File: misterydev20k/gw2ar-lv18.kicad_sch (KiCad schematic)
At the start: 53 parts, among them J3 Jumper block, U11 LY68L6400SLIT, U5 GW2AR-LV18-QN88, U6 W25Q128JVS, U8 SY8113BADC, Y2 27MHz

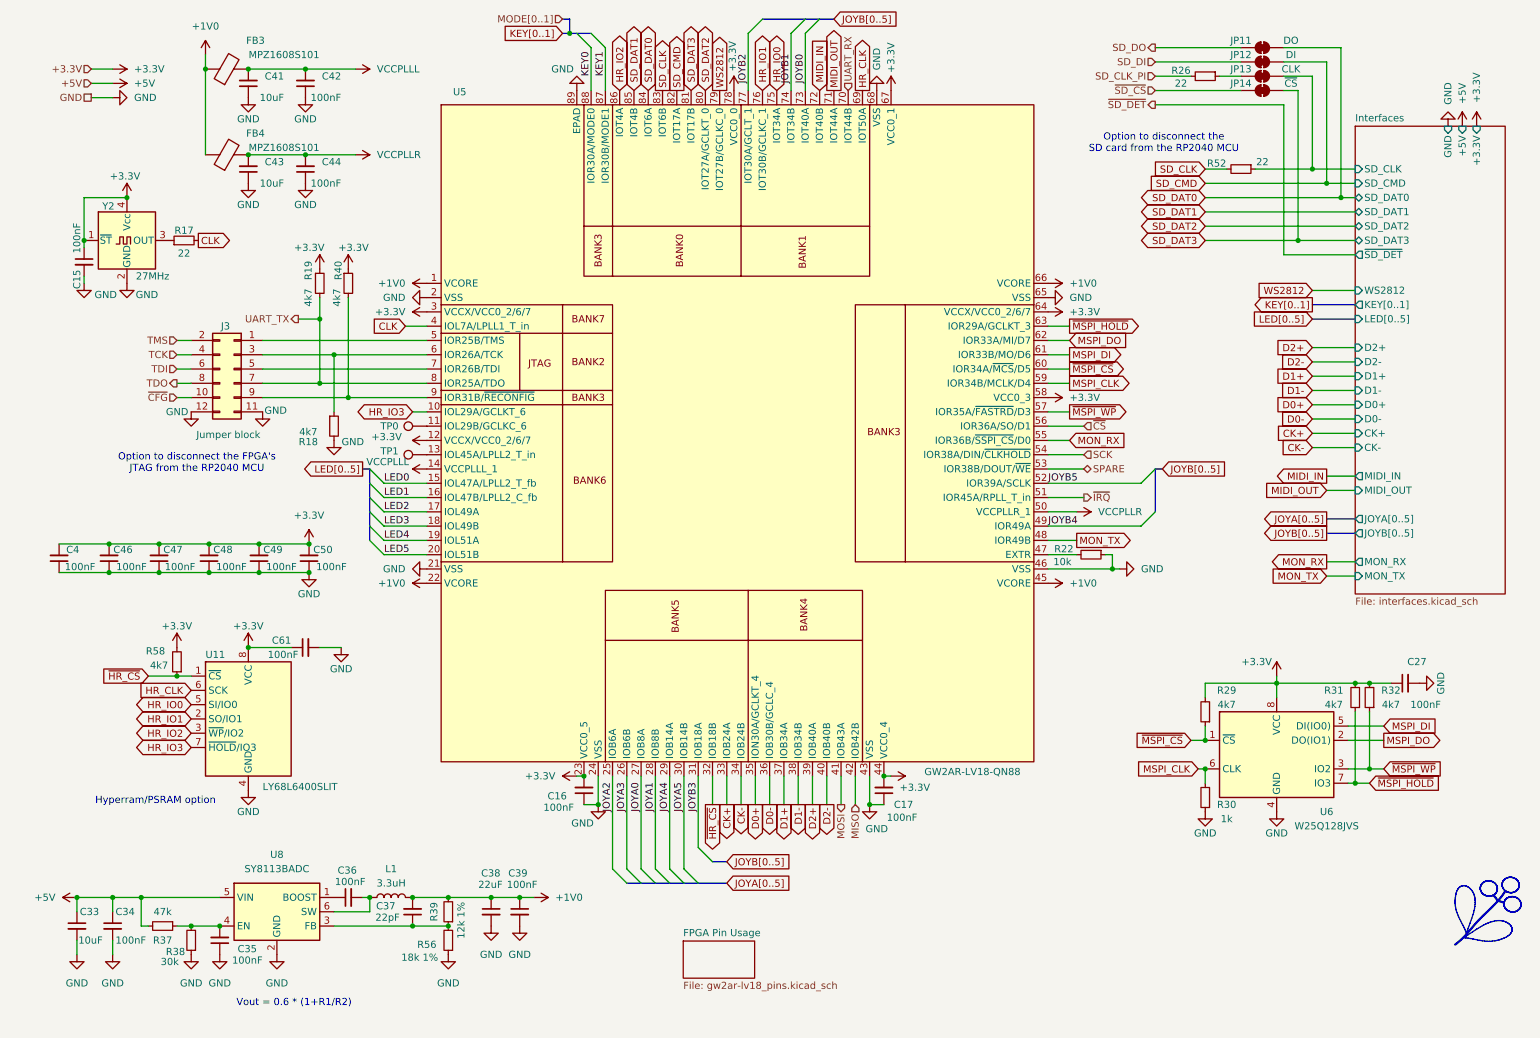
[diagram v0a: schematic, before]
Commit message: More small pcb updates
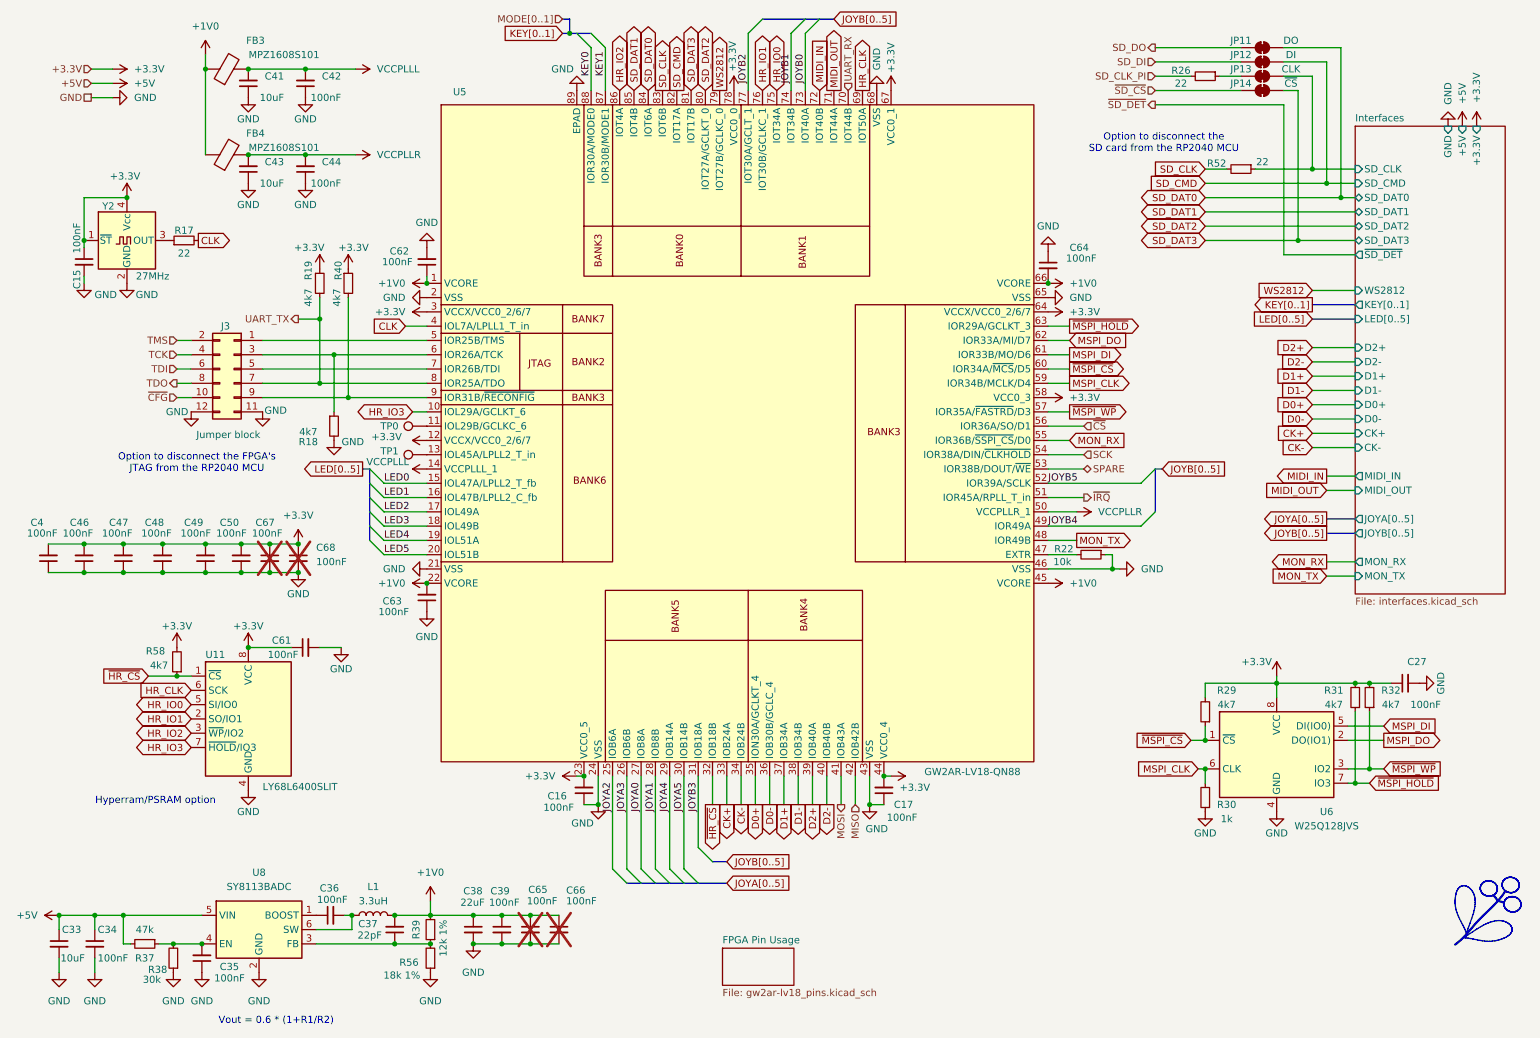
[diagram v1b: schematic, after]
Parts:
- added C62, C63, C64: 100nF, Capacitor_SMD:C_0402_1005Metric, symbol Device:C_Small
- added C65, C66, C67, C68: 100nF, Capacitor_SMD:C_0603_1608Metric, symbol Device:C_Small
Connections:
- net +1V0: now also C62.1, C63.2, C64.2, C65.1, C66.1
- net +3.3V: now also C67.1, C68.1
- net GND: now also C62.2, C63.1, C64.1, C65.2, C66.2, C67.2, C68.2
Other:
- moved on the sheet: C33, C34, C35, C36, C37, C38, C39, C4, C46, C47, C48, C49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
